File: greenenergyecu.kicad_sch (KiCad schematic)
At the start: 1 part, among them M2 Module-knock-0.2

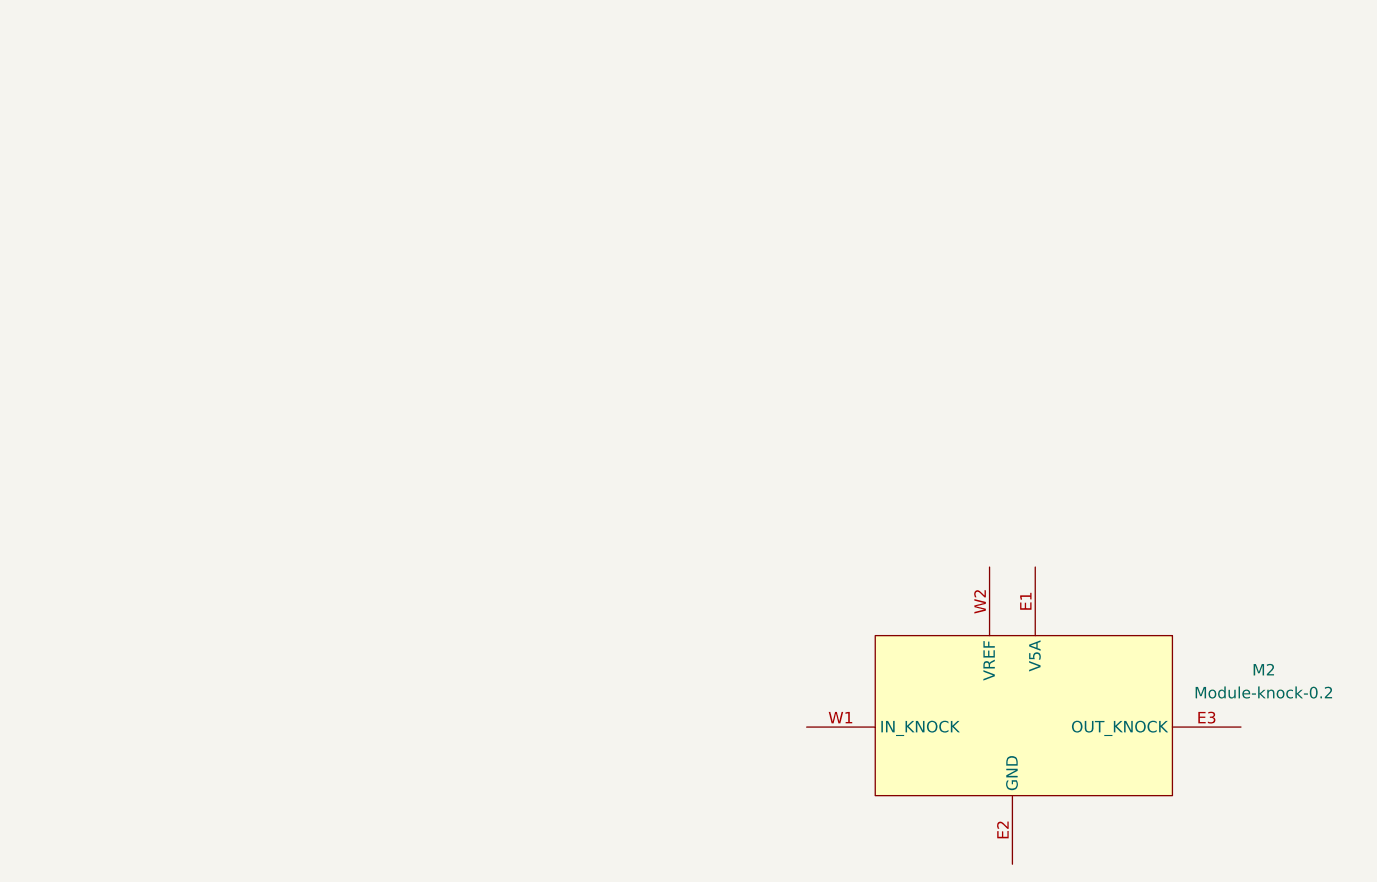
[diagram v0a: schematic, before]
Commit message: ssamklms
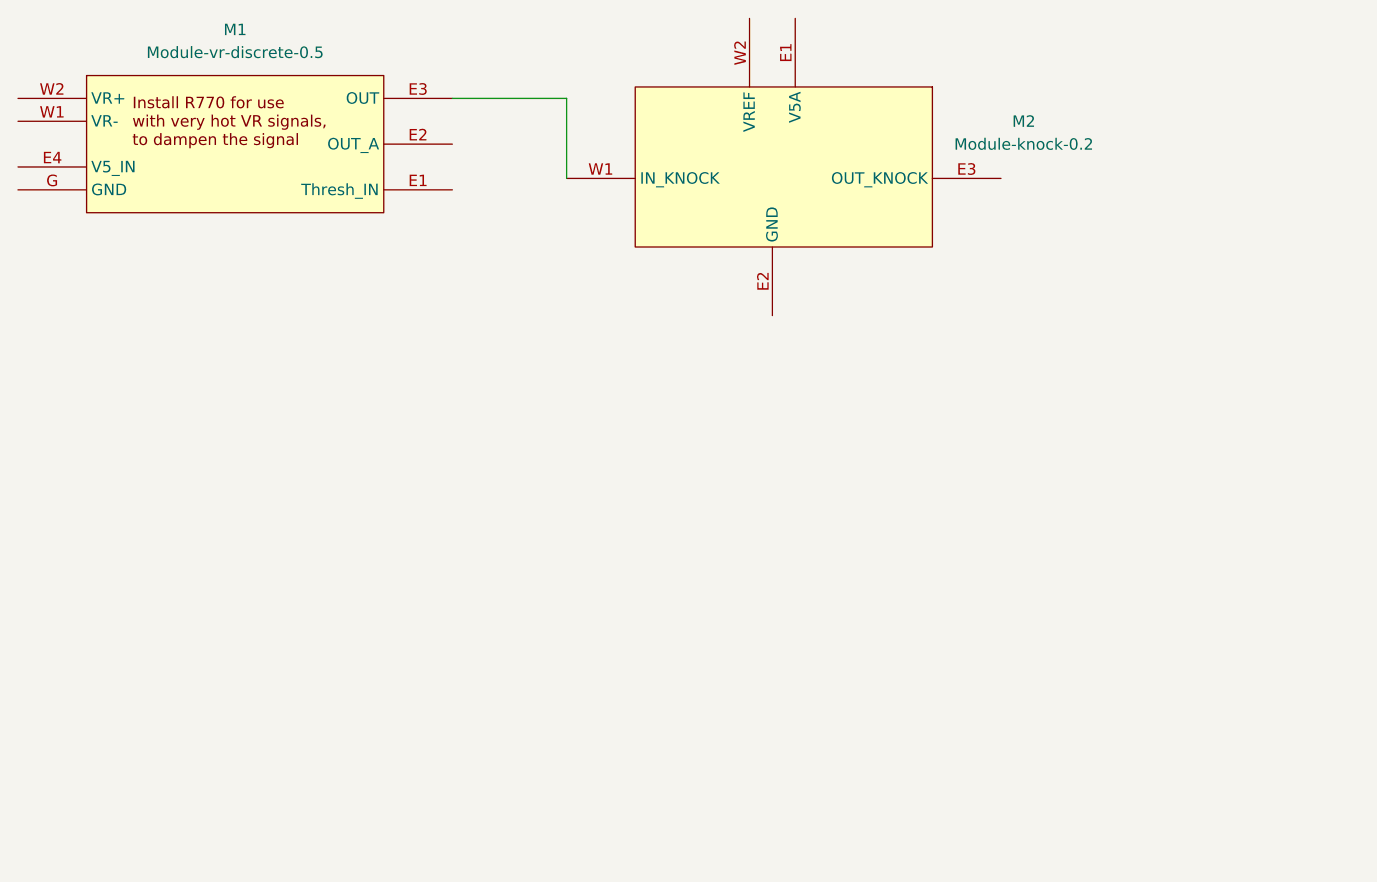
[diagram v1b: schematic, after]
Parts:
- added M1: Module-vr-discrete-0.5, hellen-one-vr-discrete-0.5:vr-discrete, symbol vr-discrete:Module-vr-discrete-0.5
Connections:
- net at M2.W1 (IN_KNOCK): now also M1.E3 (OUT)
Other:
- moved on the sheet: M2
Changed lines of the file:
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@@
 	(generator_version "8.0")
 	(paper "A4")
+	(wire
+		(pts
+			(xy 99.06 38.1) (xy 99.06 46.99)
+		)
+		(stroke
+			(width 0)
+			(type default)
+		)
+	)
+	(wire
+		(pts
+			(xy 86.36 38.1) (xy 99.06 38.1)
+		)
+		(stroke
+			(width 0)
+			(type default)
+		)
+	)
 	(symbol
 		(lib_id "knock:Module-knock-0.2")
-		(at 133.35 97.79 0)
+		(at 106.68 36.83 0)
 		(unit 1)
 		(exclude_from_sim no)
@@
 		(fields_autoplaced yes)
 		(property "Reference" "M2"
-			(at 176.53 101.6314 0)
+			(at 149.86 40.6714 0)
 			(effects
 				(font
@@
 		)
 		(property "Value" "Module-knock-0.2"
-			(at 176.53 104.1714 0)
+			(at 149.86 43.2114 0)
 			(effects
 				(font
@@
 		)
 		(property "Footprint" "hellen-one-knock-0.2:knock"
-			(at 133.35 97.79 0)
+			(at 106.68 36.83 0)
 			(effects
 				(font
@@
 		)
 		(property "Datasheet" ""
-			(at 133.35 97.79 0)
+			(at 106.68 36.83 0)
 			(effects
 				(font
@@
 		)
 		(property "Description" "Hellen-One Knock Pre-amplifier Module"
-			(at 133.35 97.79 0)
+			(at 106.68 36.83 0)
 			(effects
 				(font
@@
 					(unit 1)
 				)
+			)
+		)
+	)
+	(symbol
+		(lib_id "vr-discrete:Module-vr-discrete-0.5")
+		(at 45.72 35.56 0)
+		(unit 1)
+		(exclude_from_sim no)
+		(in_bom yes)
+		(on_board yes)
+		(dnp no)
+		(fields_autoplaced yes)
+		(property "Reference" "M1"
+			(at 62.23 30.48 0)
+			(effects
+				(font
+					(size 1.27 1.27)
+				)
+			)
+		)
+		(property "Value" "Module-vr-discrete-0.5"
+			(at 62.23 33.02 0)
+			(effects
+				(font
+					(size 1.27 1.27)
+				)
+			)
+		)
+		(property "Footprint" "hellen-one-vr-discrete-0.5:vr-discrete"
+			(at 71.12 34.29 0)
+			(effects
+				(font
+					(size 1.27 1.27)
+				)
+				(hide yes)
+			)
+		)
+		(property "Datasheet" ""
+			(at 45.72 35.56 0)
+			(effects
+				(font
+					(size 1.27 1.27)
+				)
+				(hide yes)
+			)
+		)
+		(property "Description" ""
+			(at 45.72 35.56 0)
+			(effects
+				(font
+					(size 1.27 1.27)
+				)
+				(hide yes)
+			)
+		)
+		(pin "W2"
+		)
+		(pin "W1"
+		)
+		(pin "E3"
+		)
+		(pin "E4"
+		)
+		(pin "E1"
+		)
+		(pin "E2"
+		)
+		(pin "G"
+		)
+		(instances
+			(project ""
+				(path "/21d7de3a-3085-4cf6-8b96-c28a6ef2f188"
+					(reference "M1")
+					(unit 1)
+				)
